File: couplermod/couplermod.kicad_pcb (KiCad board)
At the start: 2 copper layers, 15.2 x 12.7 mm, 6 parts, among them J1 SMA, P1 CONN_2

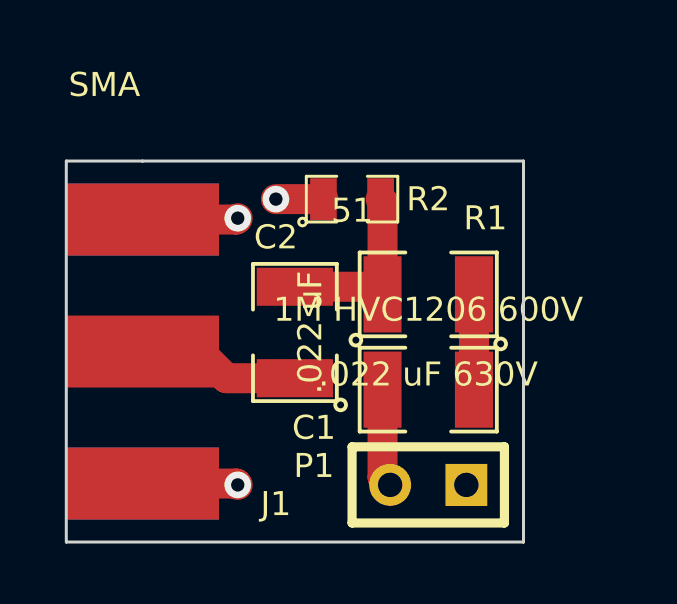
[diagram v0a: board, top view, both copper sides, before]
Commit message: cleanups to coupler mod
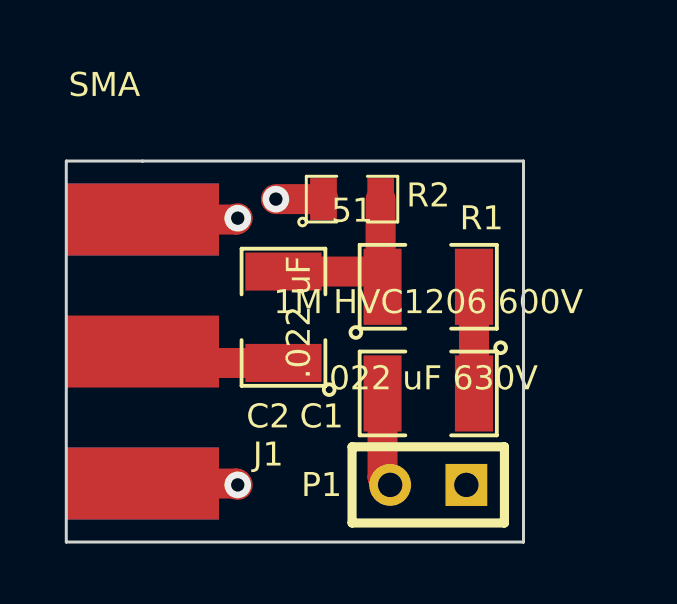
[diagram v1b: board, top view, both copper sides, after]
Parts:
- moved C2 0.63 mm to (146.3, 103.6)
- moved R1 0.25 mm to (151.1, 102.6)
- moved C1 0.13 mm to (151.1, 106.2)
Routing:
- net Net-(C2-Pad1): track 5.45 -> 6.76 mm
- net Net-(C2-Pad2): track 6.23 -> 6.76 mm
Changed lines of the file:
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@@
     (18 B.Paste user)
     (19 F.Paste user)
-    (20 B.SilkS user)
+    (20 B.SilkS user hide)
     (21 F.SilkS user)
     (22 B.Mask user)
@@
   )
   (module SMD_Packages:SMD-1210 (layer F.Cu)
-    (at 151.13 106.045 180)
+    (at 151.13 106.172 180)
     (tags "CMS SM")
     (attr smd)
-    (fp_text reference C1 (at 3.81 -1.27 180) (layer F.SilkS)
+    (fp_text reference C1 (at 3.556 -0.762 180) (layer F.SilkS)
       (effects (font (size 0.8 0.8) (thickness 0.15)))
     )
@@
   )
   (module SMD_Packages:SMD-1210 (layer F.Cu)
-    (at 146.685 104.14 90)
+    (at 146.304 103.632 90)
     (tags "CMS SM")
     (attr smd)
-    (fp_text reference C2 (at 3.175 -0.635 180) (layer F.SilkS)
+    (fp_text reference C2 (at -3.302 -0.508 180) (layer F.SilkS)
       (effects (font (size 0.8 0.8) (thickness 0.15)))
     )
@@
   (module sma:sma (layer F.Cu)
     (at 141.605 104.775)
-    (fp_text reference J1 (at 4.445 5.08) (layer F.SilkS)
+    (fp_text reference J1 (at 4.191 3.429) (layer F.SilkS)
       (effects (font (size 0.8 0.8) (thickness 0.15)))
     )
@@
     (descr "Connecteurs 2 pins")
     (tags "CONN DEV")
-    (fp_text reference P1 (at 3.81 0.635 180) (layer F.SilkS)
+    (fp_text reference P1 (at 3.556 0 180) (layer F.SilkS)
       (effects (font (size 0.8 0.8) (thickness 0.15)))
     )
@@
   )
   (module SMD_Packages:SMD-1210 (layer F.Cu)
-    (at 151.13 102.87)
+    (at 151.13 102.616)
     (tags "CMS SM")
     (attr smd)
-    (fp_text reference R1 (at 1.905 -2.54) (layer F.SilkS)
+    (fp_text reference R1 (at 1.778 -2.286) (layer F.SilkS)
       (effects (font (size 0.8 0.8) (thickness 0.15)))
     )
@@
     (at 148.59 99.695)
     (attr smd)
-    (fp_text reference R2 (at 2.54 0) (layer F.SilkS)
+    (fp_text reference R2 (at 2.54 -0.127) (layer F.SilkS)
       (effects (font (size 0.8 0.8) (thickness 0.15)))
     )
@@
     )
   )
+  (gr_text couple (at 149.86 103.505 90) (layer B.SilkS)
+    (effects (font (size 1.5 1.5) (thickness 0.3)) (justify mirror))
+  )
   (gr_text gnd (at 152.4 105.41 90) (layer B.SilkS)
-    (effects (font (size 1.5 1.5) (thickness 0.3)) (justify mirror))
-  )
-  (gr_text couple (at 149.86 103.505 90) (layer B.SilkS)
     (effects (font (size 1.5 1.5) (thickness 0.3)) (justify mirror))
   )
@@
   (gr_line (start 154.305 98.425) (end 154.305 111.125) (angle 90) (layer Edge.Cuts) (width 0.1))
   (gr_line (start 141.605 98.425) (end 154.305 98.425) (angle 90) (layer Edge.Cuts) (width 0.1))
-  (segment (start 152.654 106.045) (end 152.654 102.87) (width 1) (layer F.Cu) (net 1))
-  (segment (start 149.606 106.045) (end 149.606 108.966) (width 1) (layer F.Cu) (net 2))
-  (segment (start 149.606 108.966) (end 149.86 109.22) (width 1) (layer F.Cu) (net 2))
-  (segment (start 146.685 105.664) (end 144.399 105.664) (width 1) (layer F.Cu) (net 3))
-  (segment (start 144.399 105.664) (end 143.51 104.775) (width 1) (layer F.Cu) (net 3))
+  (segment (start 152.654 106.172) (end 152.654 102.616) (width 1) (layer F.Cu) (net 1) (status C00000))
+  (segment (start 149.606 106.172) (end 149.606 108.966) (width 1) (layer F.Cu) (net 2) (status C00000))
+  (segment (start 149.606 108.966) (end 149.86 109.22) (width 1) (layer F.Cu) (net 2) (status C00000))
+  (segment (start 146.304 105.156) (end 141.986 105.156) (width 1) (layer F.Cu) (net 3) (status C00000))
+  (segment (start 141.986 105.156) (end 141.605 104.775) (width 1) (layer F.Cu) (net 3) (status C00000))
   (segment (start 143.51 104.775) (end 141.605 104.775) (width 1) (layer F.Cu) (net 3))
-  (segment (start 149.606 102.87) (end 149.606 99.7585) (width 1) (layer F.Cu) (net 4))
-  (segment (start 149.606 99.7585) (end 149.5425 99.695) (width 1) (layer F.Cu) (net 4))
-  (segment (start 146.685 102.616) (end 149.352 102.616) (width 1) (layer F.Cu) (net 4))
-  (segment (start 149.352 102.616) (end 149.606 102.87) (width 1) (layer F.Cu) (net 4))
-  (segment (start 141.605 100.375) (end 144.735 100.375) (width 1) (layer F.Cu) (net 5) (status 400000))
+  (segment (start 149.606 102.616) (end 149.606 102.108) (width 1) (layer F.Cu) (net 4) (status C00000))
+  (segment (start 149.606 102.108) (end 146.304 102.108) (width 1) (layer F.Cu) (net 4) (status C00000))
+  (segment (start 149.5425 99.695) (end 149.5425 102.5525) (width 1) (layer F.Cu) (net 4))
+  (segment (start 149.5425 102.5525) (end 149.606 102.616) (width 1) (layer F.Cu) (net 4))
+  (via (at 146.05 99.695) (size 0.889) (layers F.Cu B.Cu) (net 5))
+  (segment (start 147.6375 99.695) (end 146.05 99.695) (width 1) (layer F.Cu) (net 5))
+  (segment (start 144.735 109.175) (end 144.78 109.22) (width 1) (layer F.Cu) (net 5))
+  (via (at 144.78 109.22) (size 0.889) (layers F.Cu B.Cu) (net 5))
+  (segment (start 141.605 109.175) (end 144.735 109.175) (width 1) (layer F.Cu) (net 5))
+  (segment (start 144.735 100.375) (end 144.78 100.33) (width 1) (layer F.Cu) (net 5))
   (via (at 144.78 100.33) (size 0.889) (layers F.Cu B.Cu) (net 5))
-  (segment (start 144.735 100.375) (end 144.78 100.33) (width 1) (layer F.Cu) (net 5))
-  (segment (start 141.605 109.175) (end 144.735 109.175) (width 1) (layer F.Cu) (net 5))
-  (via (at 144.78 109.22) (size 0.889) (layers F.Cu B.Cu) (net 5))
-  (segment (start 144.735 109.175) (end 144.78 109.22) (width 1) (layer F.Cu) (net 5))
-  (segment (start 147.6375 99.695) (end 146.05 99.695) (width 1) (layer F.Cu) (net 5))
-  (via (at 146.05 99.695) (size 0.889) (layers F.Cu B.Cu) (net 5))
+  (segment (start 141.605 100.375) (end 144.735 100.375) (width 1) (layer F.Cu) (net 5))
   (zone (net 5) (net_name GND) (layer B.Cu) (hatch edge 0.508)
     (connect_pads yes (clearance 0.5))
